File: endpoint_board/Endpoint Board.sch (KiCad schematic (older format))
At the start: 11 parts, among them P1 POWER, P4 SERIAL, P5 RUN, P6 PGRM, SW1 Switch_SPDT_x2, U1 LM3671, U2 ESP-01, U3 DotStar

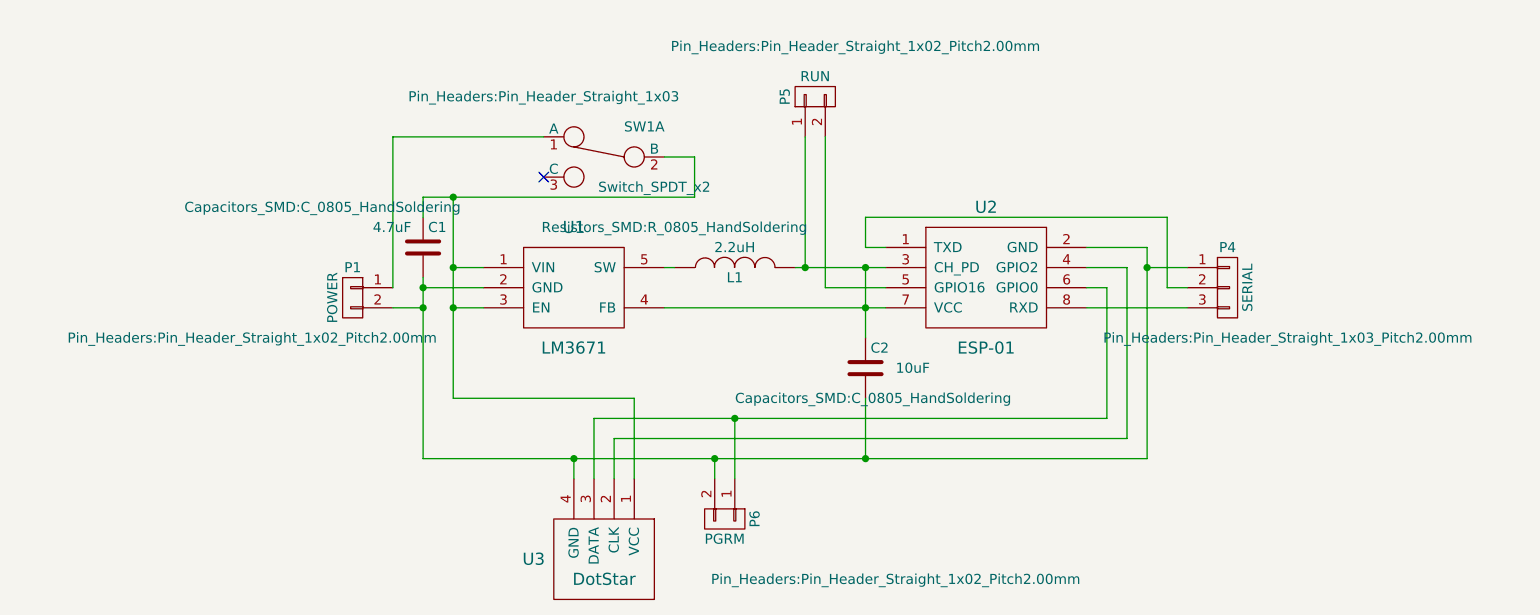
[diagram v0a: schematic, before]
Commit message: First draft of the new receivers
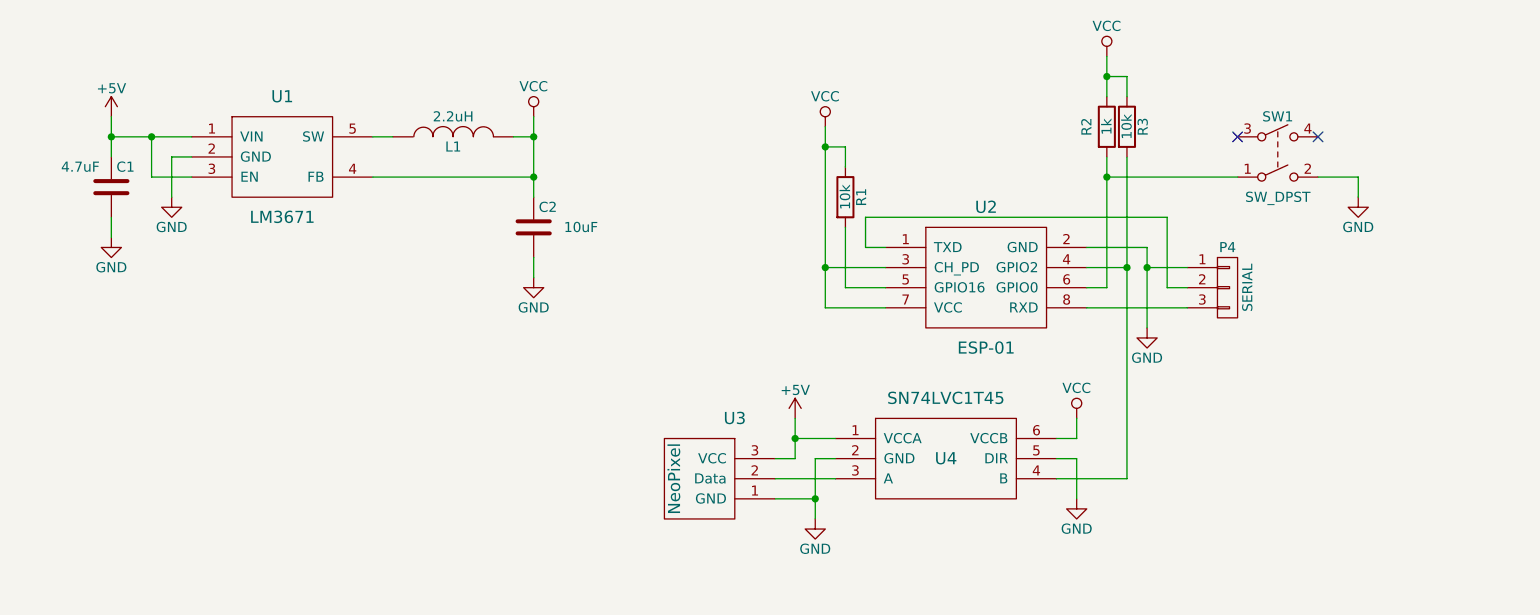
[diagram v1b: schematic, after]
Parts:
- removed P1: POWER, Pin_Headers:Pin_Header_Straight_1x02_Pitch2.00mm, symbol CONN_01X02
- removed P5: RUN, Pin_Headers:Pin_Header_Straight_1x02_Pitch2.00mm, symbol CONN_01X02
- removed P6: PGRM, Pin_Headers:Pin_Header_Straight_1x02_Pitch2.00mm, symbol CONN_01X02
- removed SW1: Switch_SPDT_x2, Pin_Headers:Pin_Header_Straight_1x03, symbol Switch_SPDT_x2
- removed U3: DotStar, symbol DotStar
- added R1, R3: 10k, Resistors_SMD:R_0805_HandSoldering, symbol R
- added R2: 1k, Resistors_SMD:R_0805_HandSoldering, symbol R
- added SW1: SW_DPST, nebrius-switch:KMR641NG, symbol SW_DPST
- added U3: NeoPixel, Pin_Headers:Pin_Header_Angled_1x03_Pitch2.54mm, symbol NeoPixel
- added U4: SN74LVC1T45, TO_SOT_Packages_SMD:TSOT-23-6_HandSoldering, symbol SN74LVC1T45
- U1: footprint (none) -> TO_SOT_Packages_SMD:SOT-23-5_HandSoldering
- U2: footprint (none) -> Pin_Headers:Pin_Header_Straight_2x04_Pitch2.54mm
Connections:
- net +5V: now reaches C1.1, U1.1 (VIN), U1.3 (EN)
- net +5V: now also U3.3 (VCC), U4.1 (VCCA)
- net GND: now reaches C1.2, C2.2, P4.1 (P1), U1.2 (GND), U2.2 (GND)
- net GND: now also SW1.2, U3.1 (GND), U4.2 (GND), U4.5 (DIR)
- net VCC: now reaches C2.1, L1.2, U1.4 (FB), U2.3 (CH_PD), U2.7 (VCC)
- net VCC: now also R1.1, R2.1, R3.1, U4.6 (VCCB)
- net at U2.5 (GPIO16): now also R1.2
- net at U2.6 (GPIO0): now also R2.2, SW1.1
- net at U2.4 (GPIO2): now also R3.2, U4.4 (B)
- new net: U3.2 (Data), U4.3 (A)
- no-connect marks 1 -> 2
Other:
- moved on the sheet: C1, C2, L1, U1
